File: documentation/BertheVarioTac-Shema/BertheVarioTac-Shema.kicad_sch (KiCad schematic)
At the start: 15 parts, among them CN1 4P-1.25 Temperature and humid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, P1 4P-1.25 Power supply base, P1 Potentiometer 10k ohms, P3 4P-1.25 Extended IO, P4 2P-1.25 SPEAK, SW1 SW_DIP_x01

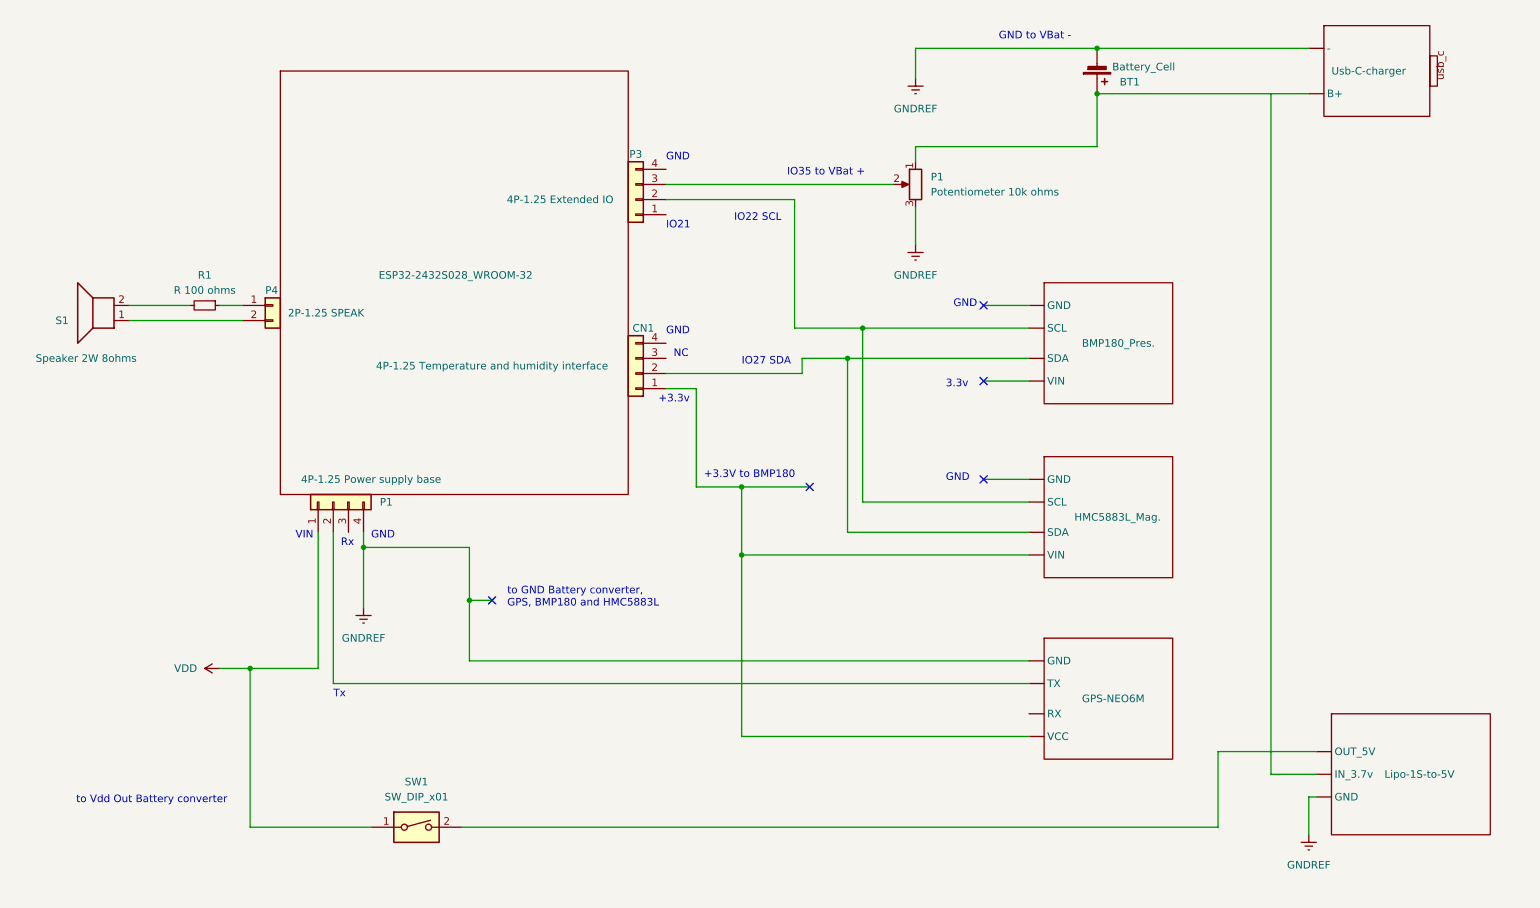
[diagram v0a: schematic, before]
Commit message: modification kicad
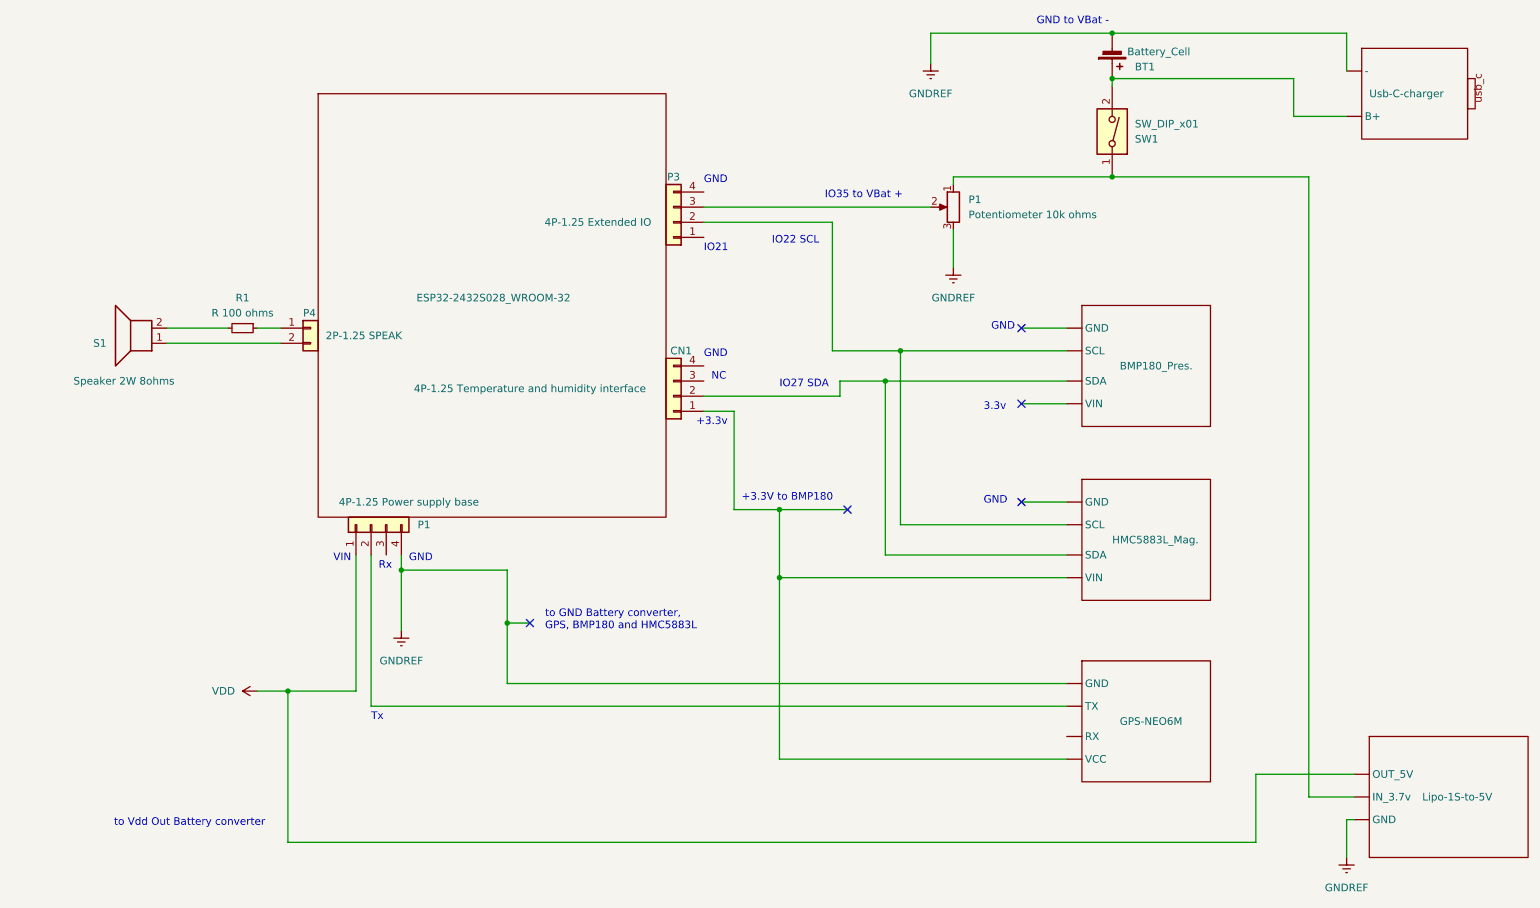
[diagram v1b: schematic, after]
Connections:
- net VDD: now also Lipo-1S-to-5V. (OUT_5V); no longer SW1.1
- net at HMC5883L_Mag.. (VIN): now also CN1.1 (Pin_1), GPS-NEO6M. (VCC)
- net at SW1.2: now also BT1.1 (+), Usb-C-charger. (B+); no longer Lipo-1S-to-5V. (OUT_5V)
- new net: BMP180_Pres.. (VIN), CN1.2 (Pin_2), HMC5883L_Mag.. (VIN)
- new net: BMP180_Pres.. (VIN), HMC5883L_Mag.. (VIN), P3.2 (Pin_2)
- new net: Lipo-1S-to-5V. (OUT_5V), P1.1, SW1.1
- now unconnected: BMP180_Pres.. (VIN), BMP180_Pres.. (VIN)
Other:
- moved on the sheet: BMP180_Pres., BT1, CN1, ESP32-2432S028_WROOM-32, GPS-NEO6M, HMC5883L_Mag., Lipo-1S-to-5V, P1, P3, P4, R1, S1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
